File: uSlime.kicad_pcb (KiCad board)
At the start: 2 copper layers, 22.1 x 27.5 mm, 29 parts, among them CN1 X1502WR-05K-N0SN, J1 USB_B_Micro, U1 ESP32-C6-MINI-1, U2 S2B-PH-K-S-GW, U3 AP2112K-3.3TRG1, U4 MCP73831T-2ACI/OT, U5 BNO085, U6 MSK-12C02_SMD_SPDT_SWITCH, Y1 32.768

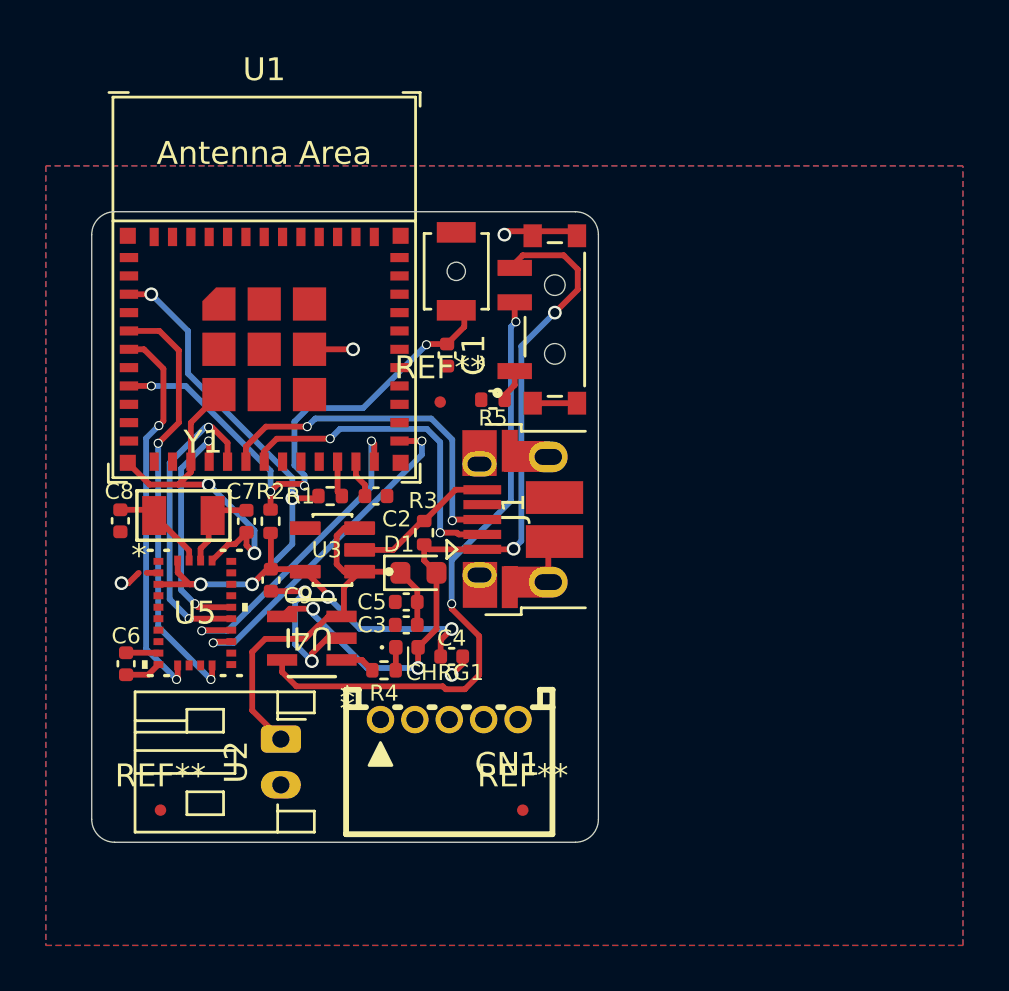
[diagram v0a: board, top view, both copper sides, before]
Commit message: Create prelim PCB
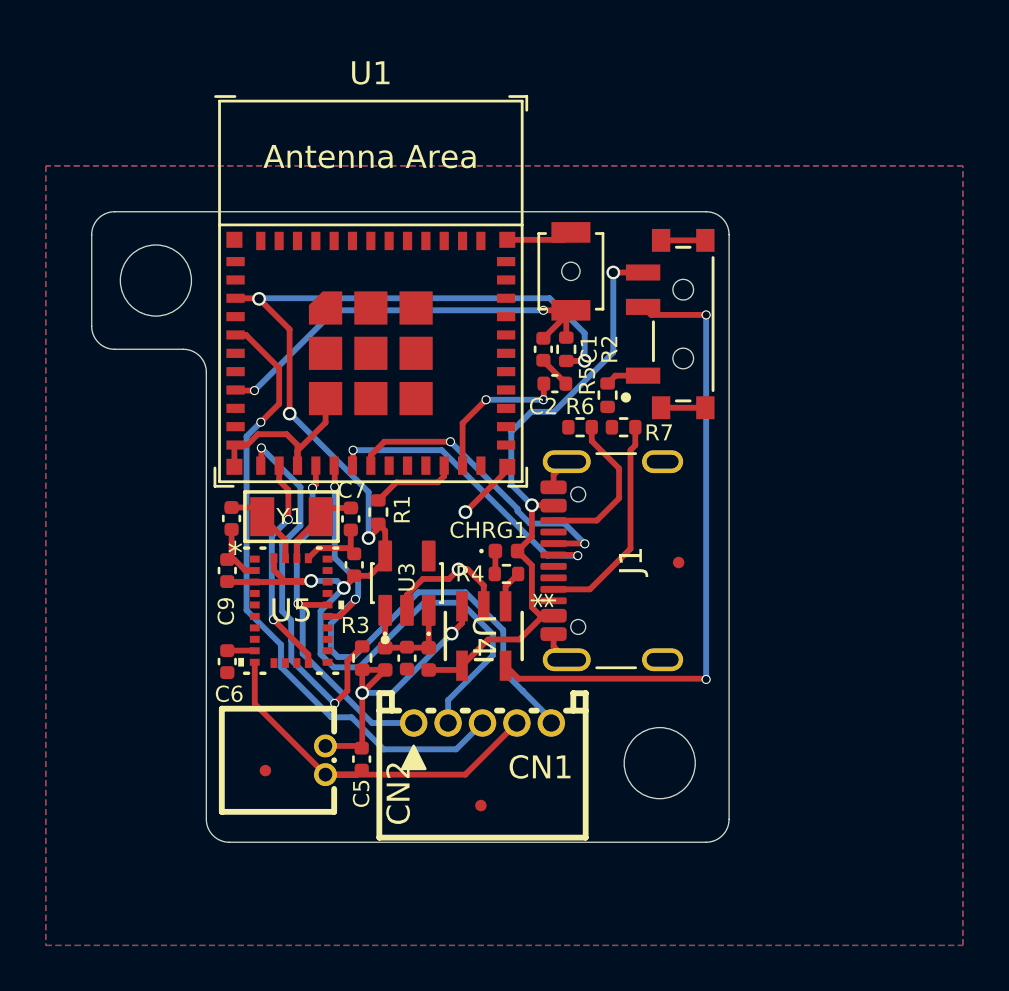
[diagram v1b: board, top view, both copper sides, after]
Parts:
- removed U2: S2B-PH-K-S-GW, Connector_JST:JST_PH_S2B-PH-K_1x02_P2.00mm_Horizontal
- added ?: , , F.Cu at (103.5, 92.3)
- added ?: , , F.Cu at (125.4, 113.4)
- added CN2: 1.25T-2AW, uSlime-libs:CONN-TH_2P-P1.25_1.25T-2AW, F.Cu at (110.8, 113.3)
- added D2: D, Diode_SMD:D_0402_1005Metric, F.Cu at (113.5, 108.8)
- added R6: 5.1k, Resistor_SMD:R_0402_1005Metric, F.Cu at (122.0, 98.8)
- added R7: 5.1k, Resistor_SMD:R_0402_1005Metric, F.Cu at (123.8, 98.8)
- C1, C2: value 0.1UF-0603-25V-(+80/-20%) -> 0.1uF
- D1: footprint Diode_SMD:D_0603_1608Metric -> Diode_SMD:D_0402_1005Metric
- J1: value USB_B_Micro -> USB_C_Receptacle_USB2.0_14P; footprint Connector_USB:USB_Micro-B_Amphenol_10103594-0001LF_Horizontal -> Connector_USB:USB_C_Receptacle_GCT_USB4105-xx-A_16P_TopMnt_Horizontal
- R3: value 100K -> 180k
- moved R2 14.9 mm to (121.3, 95.3)
- moved REF** 12.5 mm to (126.2, 104.7)
- moved C2 9.21 mm to (120.8, 96.8)
- moved U4 7.50 mm to (117.8, 107.9), turned to -90 degrees
- moved C5 7.13 mm to (112.4, 113.2), turned to 90 degrees
- moved R4 6.79 mm to (118.7, 105.2), turned to 0 degrees
- moved R3 6.10 mm to (112.5, 108.8)
- moved CHRG1 6.04 mm to (118.7, 104.2)
- moved C4 5.84 mm to (112.1, 104.8), turned to 90 degrees
- moved U6 5.60 mm to (126.5, 94.2)
- moved J1 5.34 mm to (124.5, 104.6)
- moved R5 5.00 mm to (123.2, 97.3), turned to 90 degrees
- moved RESET1 5.00 mm to (121.5, 92.0)
- moved REF** 4.89 mm to (108.2, 113.7)
- moved C8 4.85 mm to (106.8, 102.7)
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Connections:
- C3 pad 1: VBAT -> Net-(D1-K)
- CN1 pad 1: unconnected-(CN1-Pad1) -> BNO_SDA
- CN1 pad 2: unconnected-(CN1-Pad2) -> +3.3V
- CN1 pad 3: unconnected-(CN1-Pad3) -> BNO_INT2
- CN1 pad 4: unconnected-(CN1-Pad4) -> GND
- CN1 pad 5: unconnected-(CN1-Pad5) -> BNO_SCL
- D1 pad 1: VBAT -> Net-(D1-K)
- R3 pad 1: VBUS -> VBAT
- R3 pad 2: GND -> BatSense
- U1 pad 12: /ESP32-C6FH4/IO0 -> BatSense
- U1 pad 13: /ESP32-C6FH4/IO1/V_BATT_2 -> BNO_INT
- U1 pad 24: BNO_CS -> /ESP32-C6FH4/IO18/~{CS}
- U1 pad 25: BNO_MOSI -> /ESP32-C6FH4/IO19/SCK
- U1 pad 5: BNO_INT -> BNO_INT2
- U1 pad 6: BNO_RST -> /ESP32-C6FH4/IO3
- U3 pad 1: VBAT -> Net-(D1-K)
- U3 pad 3: VBAT -> Net-(D1-K)
- U5 pad 11: BNO_RST -> unconnected-(U5-NRST-Pad11)
- U5 pad 17: BNO_MOSI -> unconnected-(U5-SA0/H_MOSI-Pad17)
- U5 pad 18: BNO_CS -> unconnected-(U5-H_CSN-Pad18)
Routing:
- net BNO_INT2: track 0.00 -> 27.5 mm, vias 0 -> 1
- net +3.3V: track 37.0 -> 60.3 mm
- net BNO_RST: track 16.9 -> 0.00 mm, vias 2 -> 0
- net BatSense: track 0.00 -> 16.9 mm, vias 0 -> 2
- net BNO_MOSI: track 14.9 -> 0.00 mm, vias 2 -> 0
- net BNO_CS: track 14.3 -> 0.00 mm, vias 2 -> 0
- net BNO_SCL: track 13.3 -> 24.9 mm
- net Net-(J1-CC1): track 0.00 -> 9.48 mm
- net GND: track 41.8 -> 51.1 mm, vias 8 -> 2
- net BNO_INT: track 18.8 -> 9.74 mm
- net Net-(J1-CC2): track 0.00 -> 6.85 mm
- net VBUS: track 33.7 -> 27.7 mm, vias 4 -> 2
- net BNO_SDA: track 10.4 -> 16.1 mm
- net VBAT: track 19.0 -> 14.0 mm, vias 0 -> 2
- net /ESP32-C6FH4/IO9/BOOT: track 1.66 -> 6.51 mm, vias 0 -> 2
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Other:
- board size 22.1 x 27.5 mm -> 27.8 x 27.5 mm
